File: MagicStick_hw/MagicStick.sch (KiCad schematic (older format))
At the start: 112 parts, among them M1 MOTOR_NO_CONTACTS, Q1 MMBT2222, Q10 MMBT2222, Q11 MMBT2222, Q12 MMBT2222, Q2 IRLML6401, Q3 MMBT2222, Q4 MMBT2222, Q5 MMBT2222, Q6 LED_RGB_6PIN_PAD, Q7 LED_RGB_6PIN_PAD, Q8 MMBT2222, Q9 MMBT2222, SW1 BUTTON

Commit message: no message
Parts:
- BLN1: symbol RFICs:BALUN868JOHANSON -> RF_ICs:BALUN868JOHANSON
- DD4: symbol RFICs:CC1101 -> RF_ICs:CC1101
- XL4: PN 47491-0001 -> 105017-0001; URL (none) -> https://www.terraelectronica.ru/product/556367
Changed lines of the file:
@@
 $EndComp
 $Comp
-L RFICs:CC1101 DD4
+L RF_ICs:CC1101 DD4
 U 1 1 57197E12
 P 15600 2500
@@
 	13550 2050 14100 2050
 $Comp
-L RFICs:BALUN868JOHANSON BLN1
+L RF_ICs:BALUN868JOHANSON BLN1
 U 1 1 578CC1E9
 P 17000 1950
@@
 F 2 "Connectors:USBmicro_MOLEX_1050170001" H 1401 6931 60  0001 C CNN
 F 3 "" H 1300 -7050 60  0000 C CNN
-F 4 "47491-0001" H 1500 6550 60  0001 C CNN "PN"
+F 4 "105017-0001" H 1500 6550 60  0001 C CNN "PN"
 F 5 "9" H 1500 6550 60  0001 C CNN "SolderPoints"
 F 6 "40" H 1500 6550 60  0001 C CNN "Price"
+F 7 "https://www.terraelectronica.ru/product/556367" H 1500 6550 50  0001 C CNN "URL"
 	1    1500 6550
 	1    0    0    -1
@@
 	-1   0    0    -1
 $EndComp
+Wire Wire Line
+	18100 1850 18300 1850
 Wire Bus Line
 	14200 1350 14200 2450
-Wire Wire Line
-	18100 1850 18300 1850
 $EndSCHEMATC

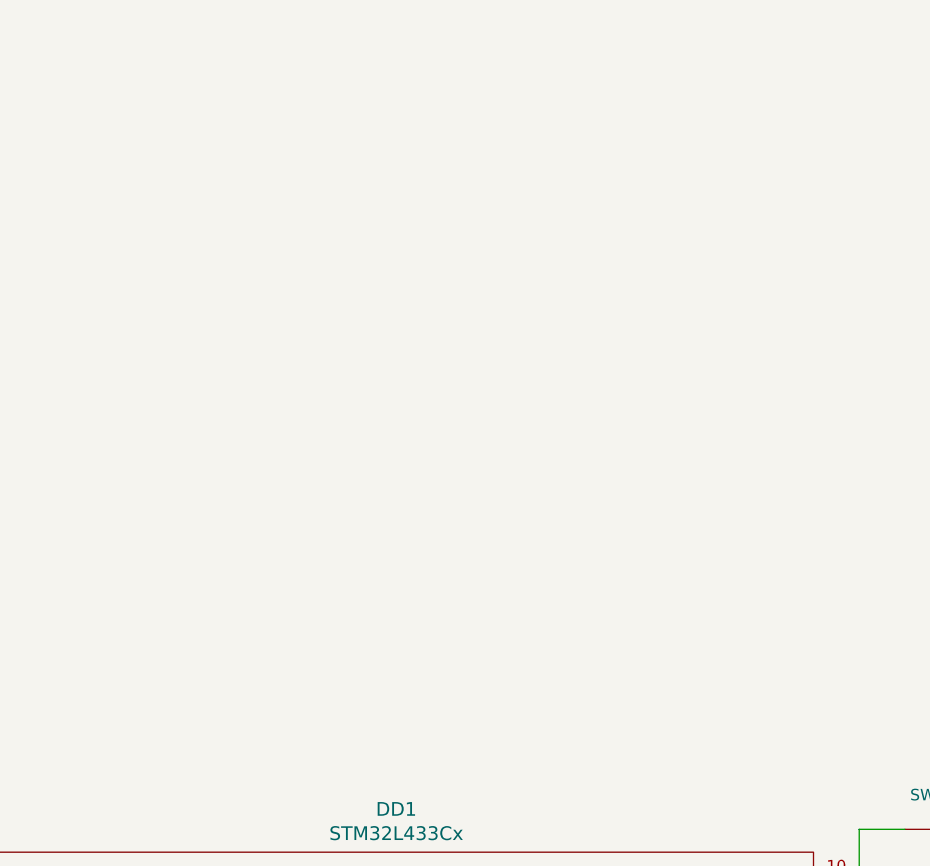
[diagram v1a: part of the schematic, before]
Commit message: + L151 code
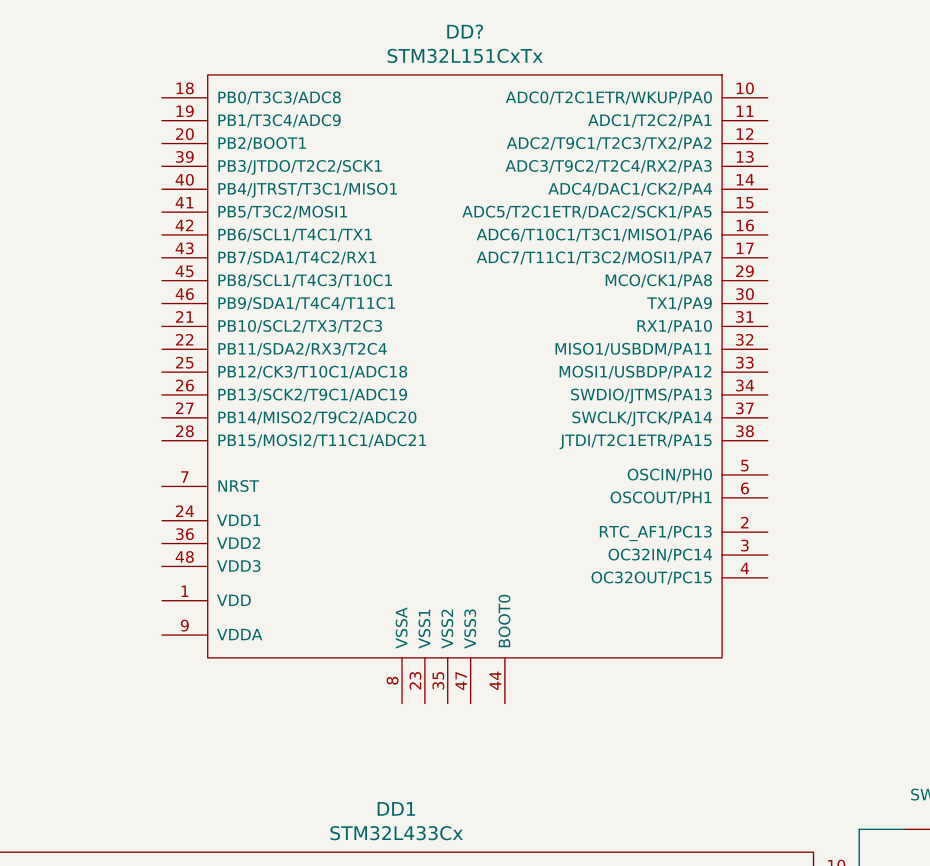
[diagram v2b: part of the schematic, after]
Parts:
- added DD?: STM32L151CxTx, LQFP_TQFP:LQFP48, symbol st_kl:STM32L151CxTx
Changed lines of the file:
@@
 Wire Bus Line
 	14200 1350 14200 2450
+$Comp
+L st_kl:STM32L151CxTx DD?
+U 1 1 5C7EBE96
+P 6850 -1200
+F 0 "DD?" H 6875 287 60  0000 C CNN
+F 1 "STM32L151CxTx" H 6875 181 60  0000 C CNN
+F 2 "LQFP_TQFP:LQFP48" H 6250 50  60  0001 C CNN
+F 3 "" H 6350 150 60  0001 C CNN
+F 4 "stm32L151c8t6" H 6450 250 60  0001 C CNN "PN"
+F 5 "http://" H 6550 350 60  0001 C CNN "URL"
+F 6 "48" H 6650 450 60  0001 C CNN "SolderPoints"
+	1    6850 -1200
+	1    0    0    -1
+$EndComp
 $EndSCHEMATC

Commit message: + L151 Avada code * CC TX race condition fixed
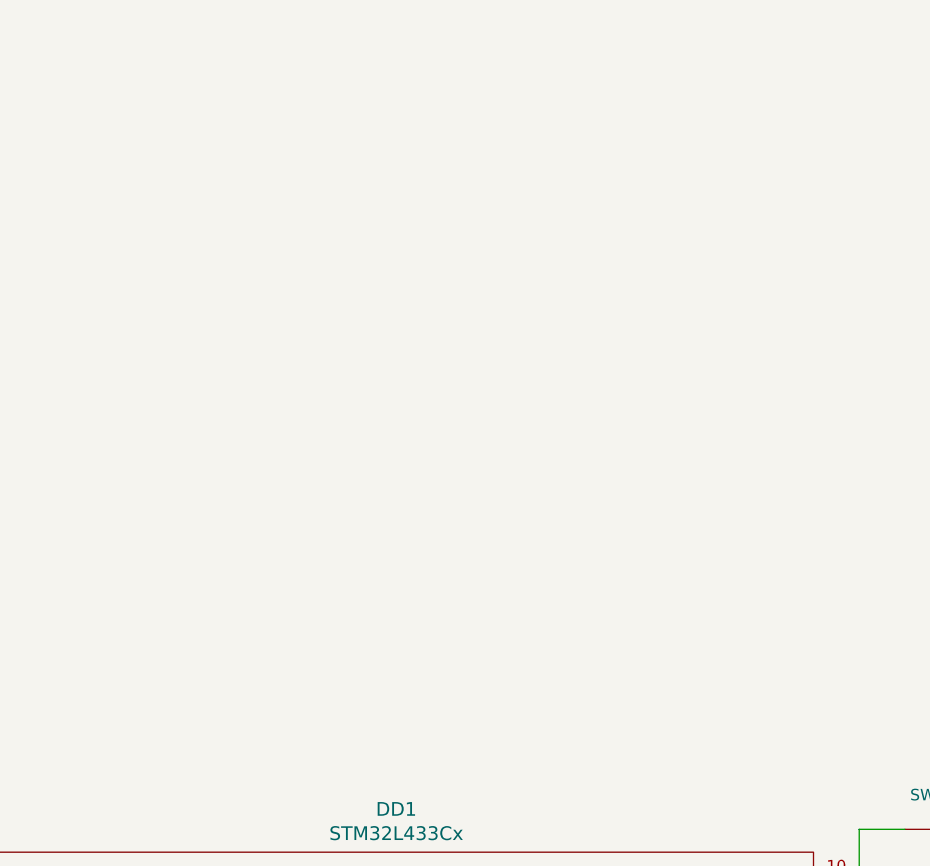
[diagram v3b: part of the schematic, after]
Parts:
- removed DD?: STM32L151CxTx, LQFP_TQFP:LQFP48, symbol st_kl:STM32L151CxTx
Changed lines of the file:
@@
 Wire Bus Line
 	14200 1350 14200 2450
-$Comp
-L st_kl:STM32L151CxTx DD?
-U 1 1 5C7EBE96
-P 6850 -1200
-F 0 "DD?" H 6875 287 60  0000 C CNN
-F 1 "STM32L151CxTx" H 6875 181 60  0000 C CNN
-F 2 "LQFP_TQFP:LQFP48" H 6250 50  60  0001 C CNN
-F 3 "" H 6350 150 60  0001 C CNN
-F 4 "stm32L151c8t6" H 6450 250 60  0001 C CNN "PN"
-F 5 "http://" H 6550 350 60  0001 C CNN "URL"
-F 6 "48" H 6650 450 60  0001 C CNN "SolderPoints"
-	1    6850 -1200
-	1    0    0    -1
-$EndComp
 $EndSCHEMATC
